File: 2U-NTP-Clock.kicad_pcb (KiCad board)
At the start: 2 copper layers, 482.6 x 87.8 mm, 279 parts, among them J1 Barrel_Jack_Switch, J2 Conn_01x06_Socket, Q1 BSS138, Q10 BSS138, Q11 BSS138, Q12 BSS138, Q13 BSS138, Q14 BSS138, Q15 BSS138, Q16 BSS138, Q17 BSS138, Q18 BSS138, Q19 BSS138, Q2 BSS138, Q20 BSS138, Q21 BSS138, Q22 BSS138, Q23 BSS138, Q24 BSS138, Q25 BSS138, Q26 BSS138, Q27 BSS138, Q28 BSS138, Q29 BSS138, Q3 BSS138, Q30 BSS138, Q31 BSS138, Q32 BSS138, Q33 BSS138, Q34 BSS138, Q35 BSS138, Q36 BSS138, Q37 BSS138, Q38 BSS138, Q39 BSS138, Q4 BSS138, Q40 BSS138, Q41 BSS138, Q42 BSS138, Q43 BSS138, Q5 BSS138, Q6 BSS138, Q7 BSS138, Q8 BSS138, Q9 BSS138, SW1 SW_Push, SW2 SW_Push, SW3 SW_Push, SW4 SW_Push, SW5 SW_Push, SW6 SW_Slide_DPDT, U3 74HC595, U4 74HC595, U5 74HC595, U6 74HC595, U7 74HC595, U8 74HC595, U9 L7805

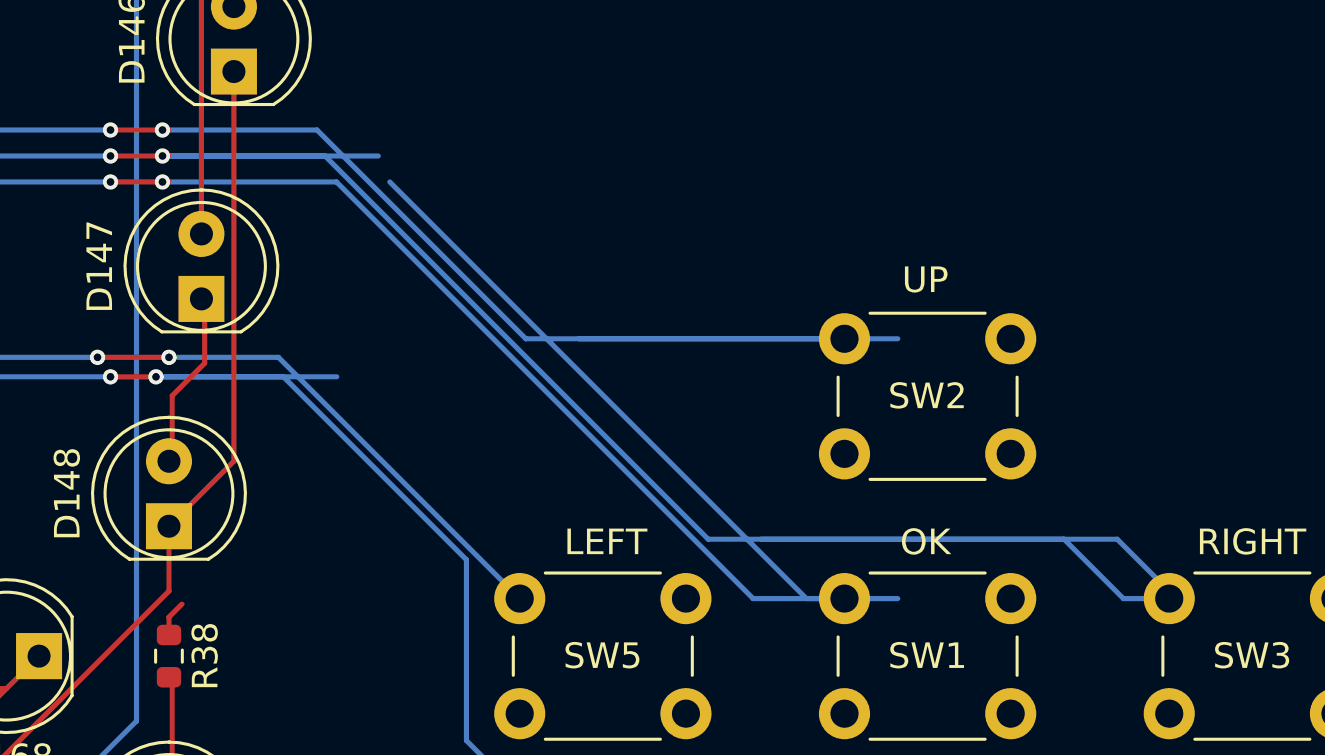
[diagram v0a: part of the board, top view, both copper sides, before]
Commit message: コンフリクト修正
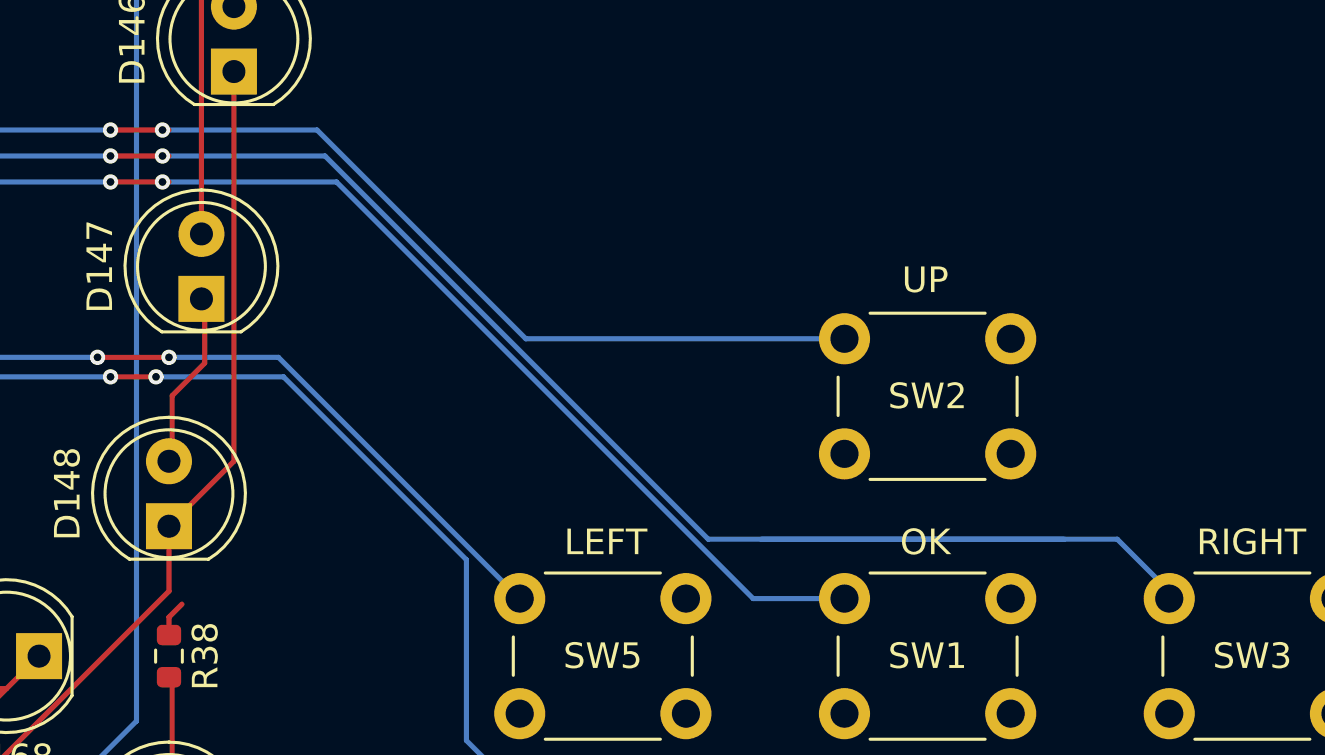
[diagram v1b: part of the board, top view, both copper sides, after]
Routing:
- net /OK: track 464.5 -> 437.9 mm
- net /RIGHT: track 478.0 -> 464.7 mm
- net /UP: track 450.1 -> 437.6 mm
- net /DOWN: track 431.8 -> 424.8 mm
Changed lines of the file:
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@@
-	)
-	(segment
-		(start 479.806 184.658)
-		(end 496.098 200.95)
-		(width 0.2)
-		(layer "B.Cu")
-		(net 3)
 	)
 	(segment
@@
 		(start 104.902 221.234)
 		(end 104.902 218.636314)
-		(width 0.2)
-		(layer "B.Cu")
-		(net 3)
-	)
-	(segment
-		(start 496.098 200.95)
-		(end 499.67 200.95)
 		(width 0.2)
 		(layer "B.Cu")
@@
 	)
 	(segment
-		(start 487.208 190.79)
-		(end 499.67 190.79)
-		(width 0.2)
-		(layer "B.Cu")
-		(net 5)
-	)
-	(segment
 		(start 468.884 182.626)
 		(end 419.1 182.626)
@@
 	)
 	(segment
-		(start 471.17 183.642)
-		(end 479.355686 183.642)
-		(width 0.2)
-		(layer "B.Cu")
-		(net 14)
-	)
-	(segment
 		(start 247.904 180.594)
 		(end 242.316 180.594)
@@
 	)
 	(segment
-		(start 506.17 198.628)
-		(end 508.492 200.95)
-		(width 0.2)
-		(layer "B.Cu")
-		(net 14)
-	)
-	(segment
 		(start 416.814 183.642)
 		(end 370.332 183.642)
@@
 	)
 	(segment
-		(start 508.492 200.95)
-		(end 510.286 200.95)
-		(width 0.2)
-		(layer "B.Cu")
-		(net 14)
-	)
-	(segment
 		(start 136.652 183.642)
 		(end 130.302 189.992)
@@
 		(width 0.2)
 		(layer "B.Cu")
-		(net 17)
-	)
-	(segment
-		(start 470.662 192.278)
-		(end 477.732314 192.278)
-		(width 0.2)
-		(layer "B.Cu")
